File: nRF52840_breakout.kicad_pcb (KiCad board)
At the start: 4 copper layers, 80 x 80 mm, 77 parts, among them J1 MM8130-2600, J2 Conn_01x12, J3 Conn_01x12, J4 Conn_01x17, J5 1734592-5, J6 Pin Header 2x5, 1.27, J7 S2B-PH-SM4-TB(LF)(SN), Q1 DMG2395, SW1 SW_Push, U1 nRF52840, U2 USB_TYPE_C, U3 AP2112K-3.3, U4 MCP73831-2-OT, Y1 32.768kHz, Y2 32MHz

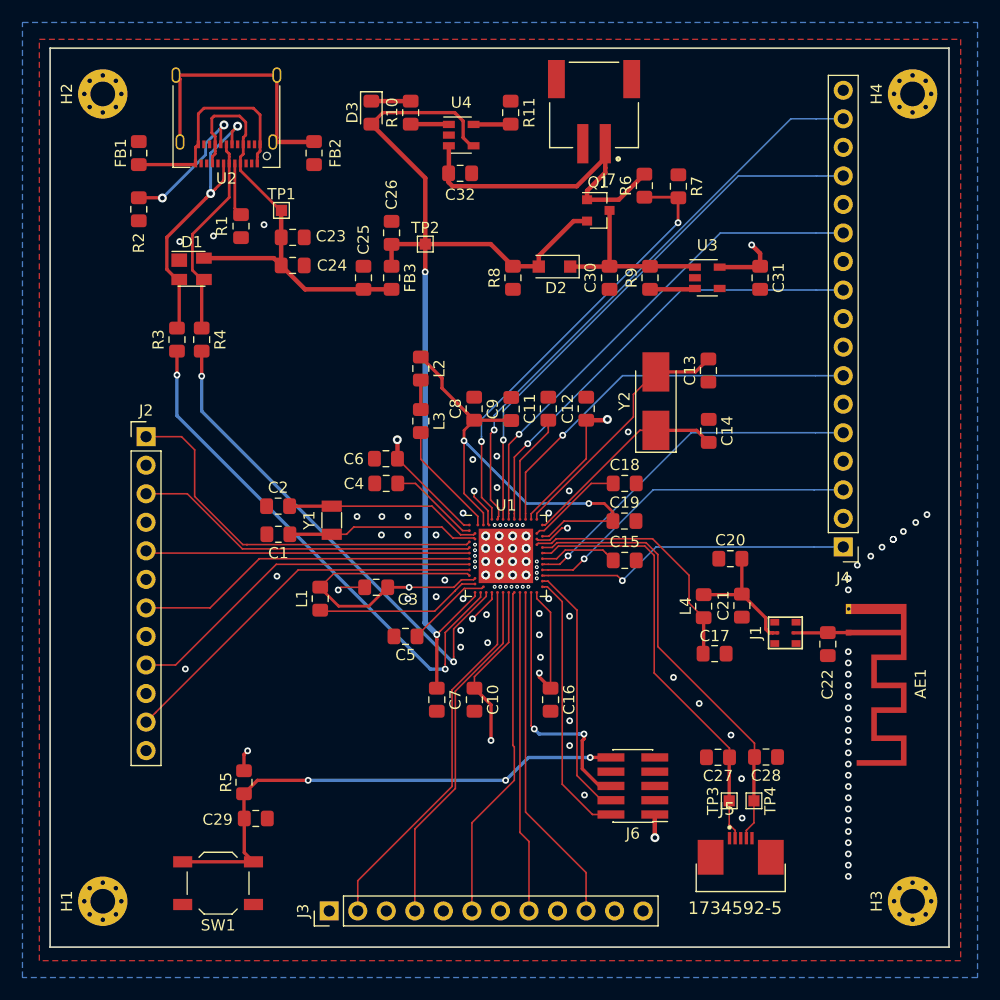
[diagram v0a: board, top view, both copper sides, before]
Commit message: added som like version of the breakout
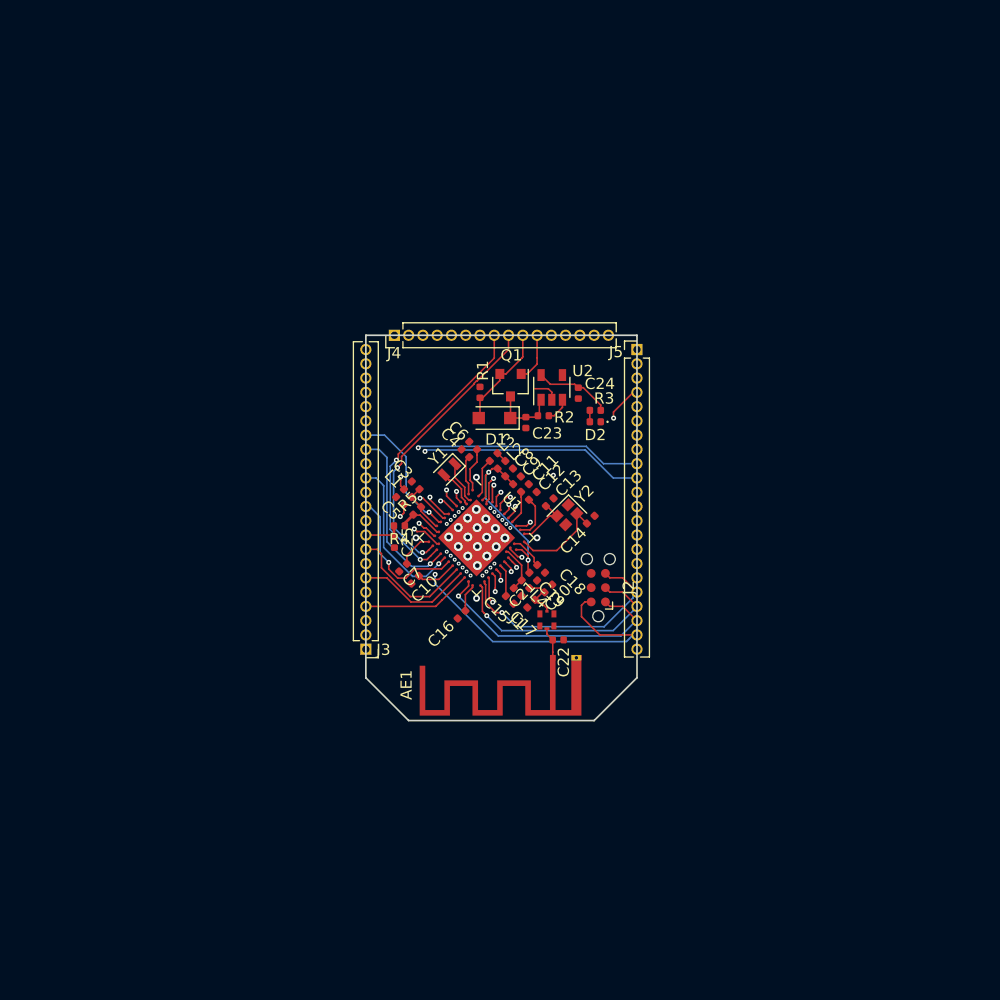
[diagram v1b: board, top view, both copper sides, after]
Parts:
- removed C1, C2: 12.5pF, Capacitor_SMD:C_0805_2012Metric_Pad1.15x1.40mm_HandSolder
- removed C26, C30, C31, C32: 10µF, Capacitor_SMD:C_0805_2012Metric_Pad1.15x1.40mm_HandSolder
- removed C27: CTUNE1, Capacitor_SMD:C_0805_2012Metric_Pad1.15x1.40mm_HandSolder
- removed C28: CTUNE2, Capacitor_SMD:C_0805_2012Metric_Pad1.15x1.40mm_HandSolder
- removed C29: 100nF, Capacitor_SMD:C_0805_2012Metric_Pad1.15x1.40mm_HandSolder
- removed D3: LED, LED_SMD:LED_0805_2012Metric_Pad1.15x1.40mm_HandSolder
- removed FB1, FB2, FB3: 120R/0.55A, Inductor_SMD:L_0805_2012Metric_Pad1.15x1.40mm_HandSolder
- removed H1, H2, H3, H4: MountingHole, MountingHole:MountingHole_2.2mm_M2_Pad_Via
- removed J6: Pin Header 2x5, 1.27, Connector_PinHeader_1.27mm:PinHeader_2x05_P1.27mm_Vertical_SMD
- removed J7: S2B-PH-SM4-TB(LF)(SN), custom_footprints:JST_PH_S2B-PH-SM4-TB_LF__SN_
- removed R10, R6, R7, R8, R9: 100k, Resistor_SMD:R_0805_2012Metric_Pad1.15x1.40mm_HandSolder
- removed R11: 5k, Resistor_SMD:R_0805_2012Metric_Pad1.15x1.40mm_HandSolder
- removed SW1: SW_Push, Button_Switch_SMD:SW_SPST_TL3342
- removed TP1: VBUS_Raw, TestPoint:TestPoint_Pad_1.0x1.0mm
- removed TP2: VBUS_nRF, TestPoint:TestPoint_Pad_1.0x1.0mm
- removed TP3: NFC1, TestPoint:TestPoint_Pad_1.0x1.0mm
- removed TP4: NFC2, TestPoint:TestPoint_Pad_1.0x1.0mm
- removed U3: AP2112K-3.3, Package_TO_SOT_SMD:SOT-23-5
- removed U4: MCP73831-2-OT, Package_TO_SOT_SMD:SOT-23-5
- C10, C11, C12, C15, C16, C17, C18, C19, C20, C21, C22, C23, C24, C3, C4, C5, C6, C7, C8, C9: footprint Capacitor_SMD:C_0805_2012Metric_Pad1.15x1.40mm_HandSolder -> Capacitor_SMD:C_0402_1005Metric
- C13, C14: value 8pF -> 6pF; footprint Capacitor_SMD:C_0805_2012Metric_Pad1.15x1.40mm_HandSolder -> Capacitor_SMD:C_0402_1005Metric
- C25: value 100nF -> NC; footprint Capacitor_SMD:C_0805_2012Metric_Pad1.15x1.40mm_HandSolder -> Capacitor_SMD:C_0402_1005Metric
- D1: value PRTR5V0U2X -> MBR120; footprint Package_TO_SOT_SMD:SOT-143 -> Diode_SMD:D_SOD-123F
- D2: value MBR120 -> LED_RED; footprint Diode_SMD:D_SOD-123F -> LED_SMD:LED_0402_1005Metric
- J1: value MM8130-2600 -> MM8930_2620; footprint custom_footprints:COAX_MM8130-2600 -> custom_footprints:MM8930_2620
- J2: value Conn_01x12 -> Conn_02x03_Odd_Even; footprint Connector_PinHeader_2.54mm:PinHeader_1x12_P2.54mm_Vertical -> Connector:Tag-Connect_TC2030-IDC-NL_2x03_P1.27mm_Vertical
- J3: value Conn_01x12 -> Conn_01x22; footprint Connector_PinHeader_2.54mm:PinHeader_1x12_P2.54mm_Vertical -> Connector_PinHeader_1.27mm:PinHeader_1x22_P1.27mm_Vertical
- J4: value Conn_01x17 -> Conn_01x16; footprint Connector_PinHeader_2.54mm:PinHeader_1x17_P2.54mm_Vertical -> Connector_PinHeader_1.27mm:PinHeader_1x16_P1.27mm_Vertical
- J5: value 1734592-5 -> Conn_01x22; footprint custom_footprints:CONNECTOR_FFC_1734592-5 -> Connector_PinHeader_1.27mm:PinHeader_1x22_P1.27mm_Vertical
- L1: value 10µH -> NC; footprint Inductor_SMD:L_0805_2012Metric_Pad1.15x1.40mm_HandSolder -> Inductor_SMD:L_0402_1005Metric
- L2, L3, L4: footprint Inductor_SMD:L_0805_2012Metric_Pad1.15x1.40mm_HandSolder -> Inductor_SMD:L_0402_1005Metric
- R1, R2: value 5.1k -> 100k; footprint Resistor_SMD:R_0805_2012Metric_Pad1.15x1.40mm_HandSolder -> Resistor_SMD:R_0402_1005Metric
- R3: value 22 -> 1k; footprint Resistor_SMD:R_0805_2012Metric_Pad1.15x1.40mm_HandSolder -> Resistor_SMD:R_0402_1005Metric
- R4: value 22 -> NC; footprint Resistor_SMD:R_0805_2012Metric_Pad1.15x1.40mm_HandSolder -> Resistor_SMD:R_0402_1005Metric
- R5: value 10k -> 0R; footprint Resistor_SMD:R_0805_2012Metric_Pad1.15x1.40mm_HandSolder -> Resistor_SMD:R_0402_1005Metric
- U2: value USB_TYPE_C -> AP2112K-3.3; footprint custom_footprints:USB_C_Receptacle_Amphenol_12401610E4-2A -> Package_TO_SOT_SMD:SOT-23-5
- Y1: value 32.768kHz -> 32.768kHz-SIT1533AI-H4-DCC-32.768E; footprint Crystal:Crystal_SMD_3215-2Pin_3.2x1.5mm -> Crystal:Crystal_SMD_2012-2Pin_2.0x1.2mm
- Y2: value 32MHz -> 32MHz-XRCGB32M000F1H00R0; footprint Crystal:Crystal_SMD_5032-2Pin_5.0x3.2mm_HandSoldering -> Crystal:Crystal_SMD_2016-4Pin_2.0x1.6mm
- moved J5 47.0 mm to (123.2, 54.6)
- moved J4 44.2 mm to (101.6, 53.3), turned to 90 degrees
- moved J2 42.4 mm to (119.8, 75.8), turned to 90 degrees
- moved R2 40.4 mm to (114.9, 60.5), turned to 180 degrees
- moved U2 38.2 mm to (115.6, 58.0), turned to 90 degrees
- moved R3 37.8 mm to (119.5, 60.0), turned to 180 degrees
- moved D1 30.1 mm to (110.5, 60.7), turned to 180 degrees
- moved R5 28.7 mm to (103.6, 69.0), turned to 45 degrees
- moved C24 27.8 mm to (118.0, 58.5), turned to 270 degrees
- moved C23 26.5 mm to (113.3, 61.1), turned to 270 degrees
- moved AE1 26.4 mm to (115.7, 82.0), turned to 180 degrees
- moved R1 25.9 mm to (109.2, 58.4), turned to 270 degrees
- moved R4 24.2 mm to (102.0, 70.3), turned to 180 degrees
- moved C22 24.0 mm to (116.2, 80.5), turned to 0 degrees
- moved C25 23.7 mm to (101.6, 71.8), turned to 270 degrees
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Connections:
- C24 pad 1: Net-(C23-Pad1) -> VDD_nRF
- C25 pad 1: Net-(C23-Pad1) -> VDDH
- D1 pad 1: GND -> Net-(C23-Pad1)
- D1 pad 2: Net-(D1-Pad2) -> VBUS_nRF
- D2 pad 1: Net-(C30-Pad1) -> GND
- D2 pad 2: VBUS_nRF -> Net-(D2-Pad2)
- J2 pad 1: P0.26 -> P1.00_SWO
- J2 pad 2: P0.27 -> P1.18_RESET
- J2 pad 3: P0.04_AIN2 -> SWDIO
- J2 pad 4: P0.05_AIN3 -> GND
- J2 pad 5: P0.06 -> SWDCLK
- J2 pad 6: P0.07 -> VDD_nRF
- J3 pad 1: P0.14 -> GND
- J3 pad 10: P0.24 -> P0.19
- J3 pad 11: P0.25 -> P0.17
- J3 pad 12: P1.01 -> P0.16
- J3 pad 2: P0.15 -> VDD_nRF
- J3 pad 3: P0.16 -> P0.25
- J3 pad 4: P0.17 -> P0.24
- J3 pad 5: P0.19 -> P0.23
- J3 pad 6: P0.20 -> P0.22
- J3 pad 8: P0.22 -> P0.20
- J3 pad 9: P0.23 -> VDDH
- J4 pad 1: P1.02 -> P0.07
- J4 pad 10: P1.13 -> VBUS_nRF
- J4 pad 11: P1.14 -> VDD_BAT
- J4 pad 12: P1.15 -> P0.31_AIN7
- J4 pad 13: P0.03_AIN1 -> P0.30_AIN6
- J4 pad 14: P0.02_AIN0 -> P0.29_AIN5
- J4 pad 16: P0.29_AIN5 -> P0.02_AIN0
- J4 pad 2: P1.03 -> P0.06
- J4 pad 3: P1.04 -> P0.05_AIN3
- J4 pad 4: P1.05 -> P0.04_AIN2
- J4 pad 5: P1.06 -> P0.27
- J4 pad 6: P1.07 -> P0.26
- J4 pad 7: P1.10 -> GND
- J4 pad 8: P1.11 -> D+
- J4 pad 9: P1.12 -> D-
- J5 pad 1: Net-(J5-Pad1) -> GND
- J5 pad 2: P0.09_NFC1 -> VDD_nRF
- J5 pad 3: Net-(J5-Pad3) -> P1.15
- J5 pad 4: P0.10_NFC2 -> P1.14
- J5 pad 5: Net-(J5-Pad5) -> P1.13
- Q1 pad 3: Net-(C30-Pad1) -> Net-(C23-Pad1)
- R1 pad 2: Net-(R1-Pad2) -> VBUS_nRF
- R2 pad 1: GND -> Net-(R2-Pad1)
- R2 pad 2: Net-(R2-Pad2) -> Net-(C23-Pad1)
- R3 pad 1: D- -> VDD_nRF
- R3 pad 2: Net-(D1-Pad2) -> Net-(D2-Pad2)
- R4 pad 1: Net-(D1-Pad3) -> Net-(R4-Pad1)
- R4 pad 2: D+ -> VDDH
- R5 pad 1: VDD_nRF -> Net-(R4-Pad1)
- R5 pad 2: P1.18_RESET -> VDD_nRF
- U1 pad Y2: VDD_nRF -> Net-(R4-Pad1)
- Y2 pad 1: Net-(C14-Pad2) -> GND
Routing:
- net VBUS_nRF: track 91.8 -> 12.4 mm, vias 2 -> 0
- net VDD_nRF: track 88.3 -> 25.6 mm, vias 8 -> 0
- net Net-(C23-Pad1): track 44.8 -> 6.02 mm
- net P0.30_AIN6: track 55.1 -> 17.8 mm
- net P0.29_AIN5: track 51.7 -> 17.9 mm
- net P1.18_RESET: track 63.9 -> 30.4 mm, vias 4 -> 2
- net VDD_BAT: track 37.2 -> 4.00 mm
- net P0.28_AIN4: track 50.0 -> 19.1 mm
- net P0.02_AIN0: track 48.6 -> 19.4 mm
- net Net-(C19-Pad1): track 45.8 -> 17.9 mm
- net P1.15: track 44.2 -> 17.5 mm
- net Net-(D1-Pad2): track 26.2 -> 0.00 mm, vias 2 -> 0
- net P1.14: track 43.1 -> 16.9 mm, vias 1 -> 2
- net P1.13: track 41.0 -> 15.5 mm
- net Net-(FB2-Pad2): track 24.9 -> 0.00 mm
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- removed copper zone on B.Cu, net GND
- removed copper zone on F.Cu, net GND
- removed copper zone on In1.Cu, net GND
- removed copper zone on In2.Cu, net VDD_nRF
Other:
- board size 80 x 80 mm -> 24.1 x 34.3 mm
- net class custom: via_dia 0.61 -> 0.45; via_drill 0.305 -> 0.2
- rule via_min_drill: 0.3 -> 0.2
- rule via_min_size: 0.4 -> 0.45
